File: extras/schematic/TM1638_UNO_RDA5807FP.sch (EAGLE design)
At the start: 10 parts, among them IC1 TM1638, Q1 32768k

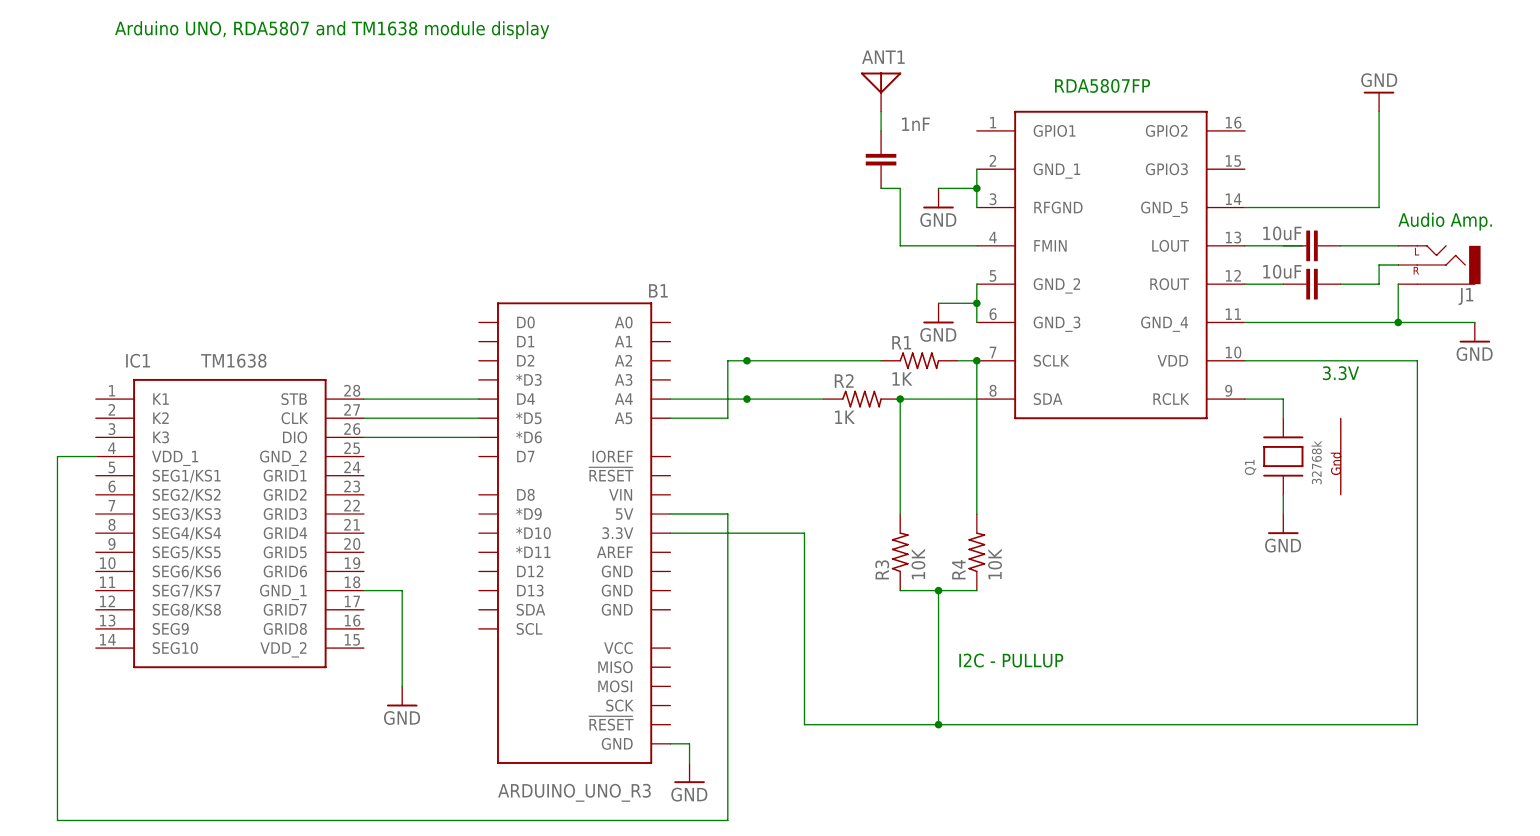
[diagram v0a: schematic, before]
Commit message: Documentation
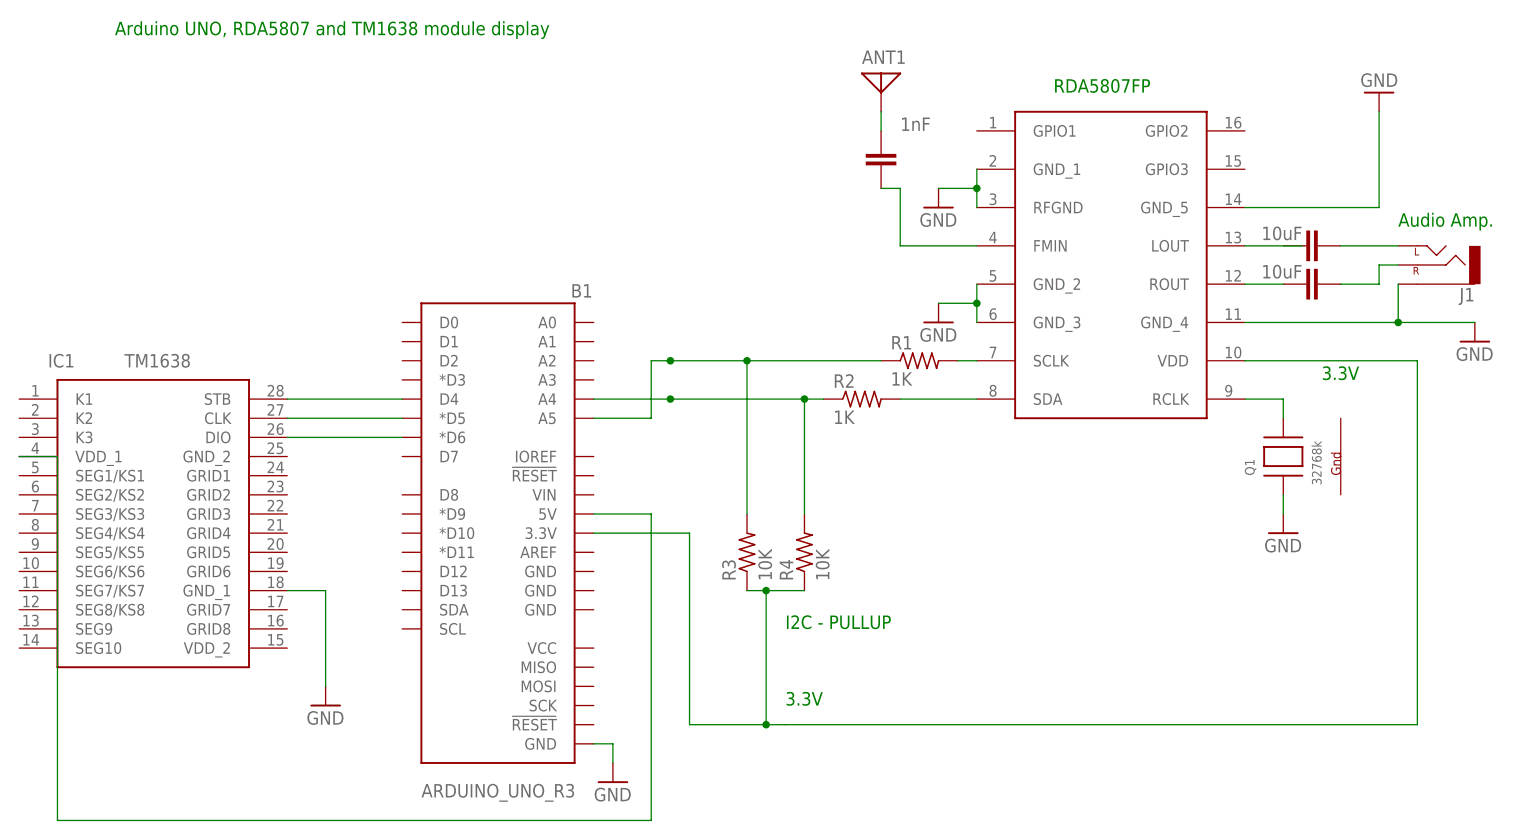
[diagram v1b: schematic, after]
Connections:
- net N$1: no longer R4.2
- net N$2: no longer R3.2
- net N$4: now also R3.2
- net N$5: now also R4.2
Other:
- moved on the sheet: B1, IC1, R3, R4
